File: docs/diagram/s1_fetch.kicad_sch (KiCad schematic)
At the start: 0 parts

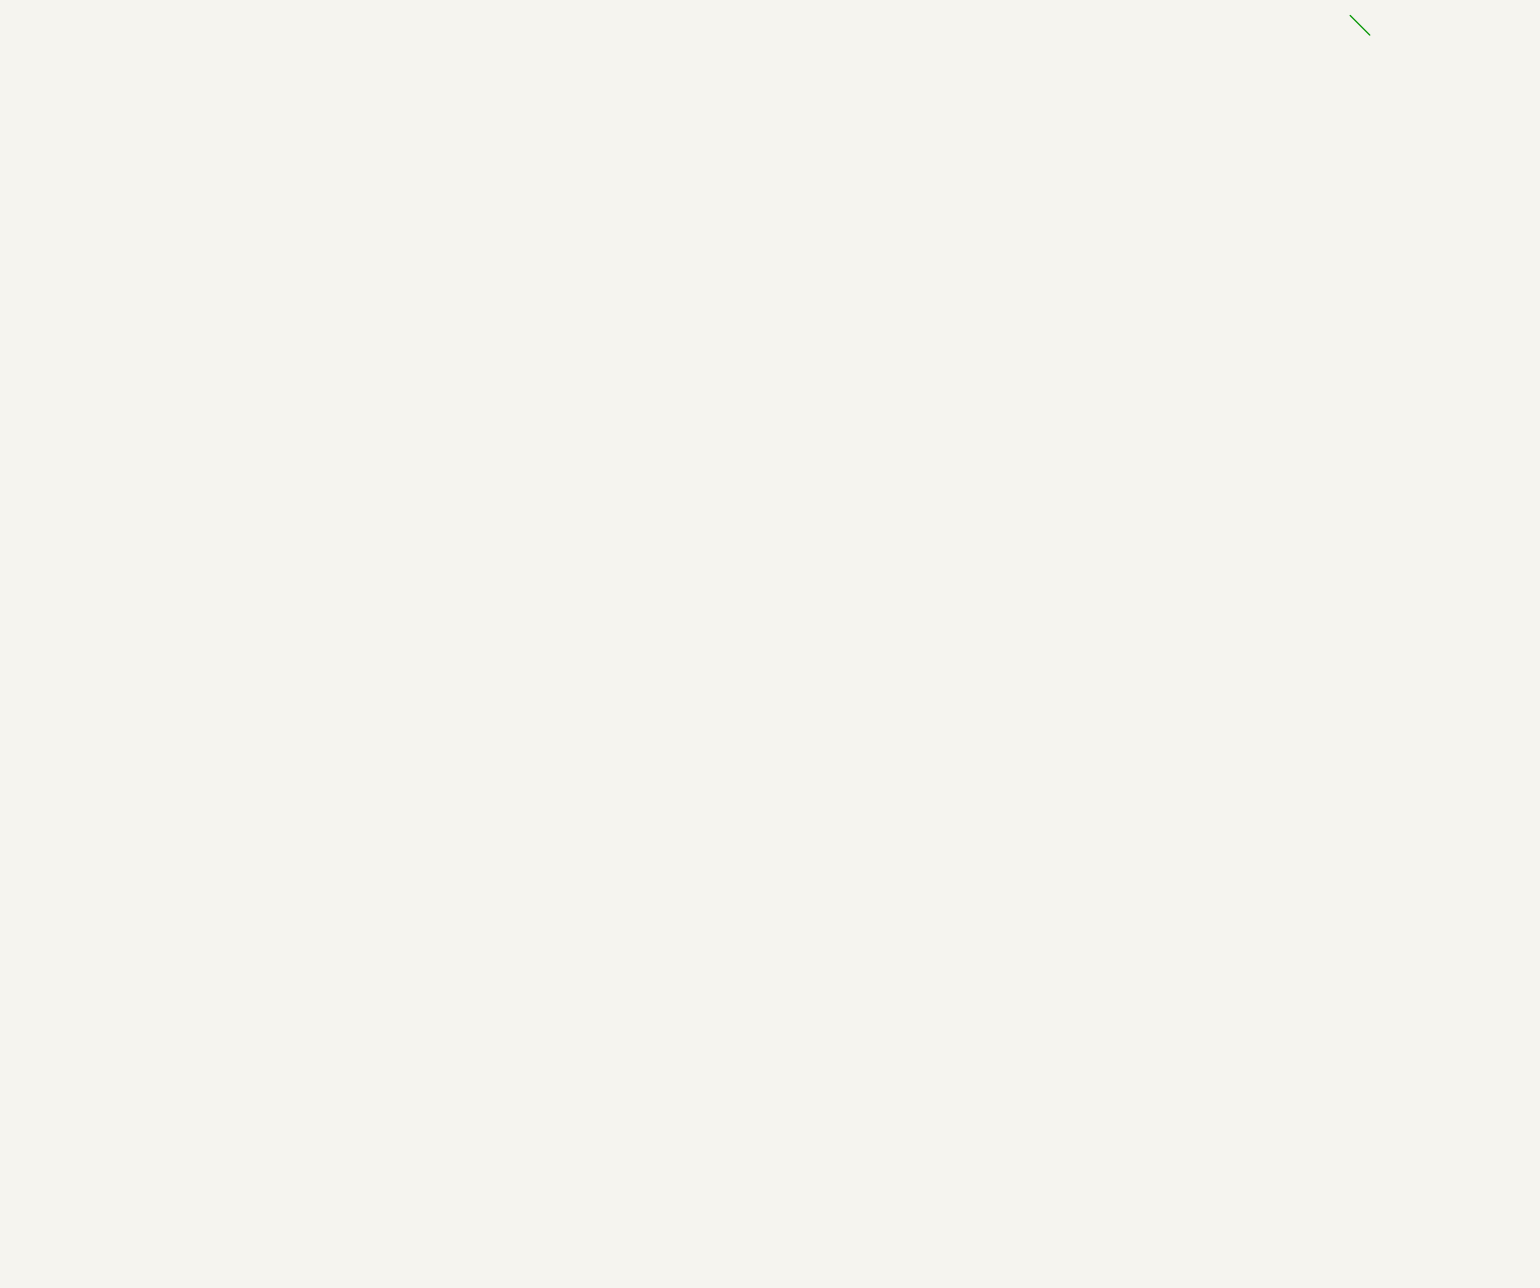
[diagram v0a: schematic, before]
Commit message: push
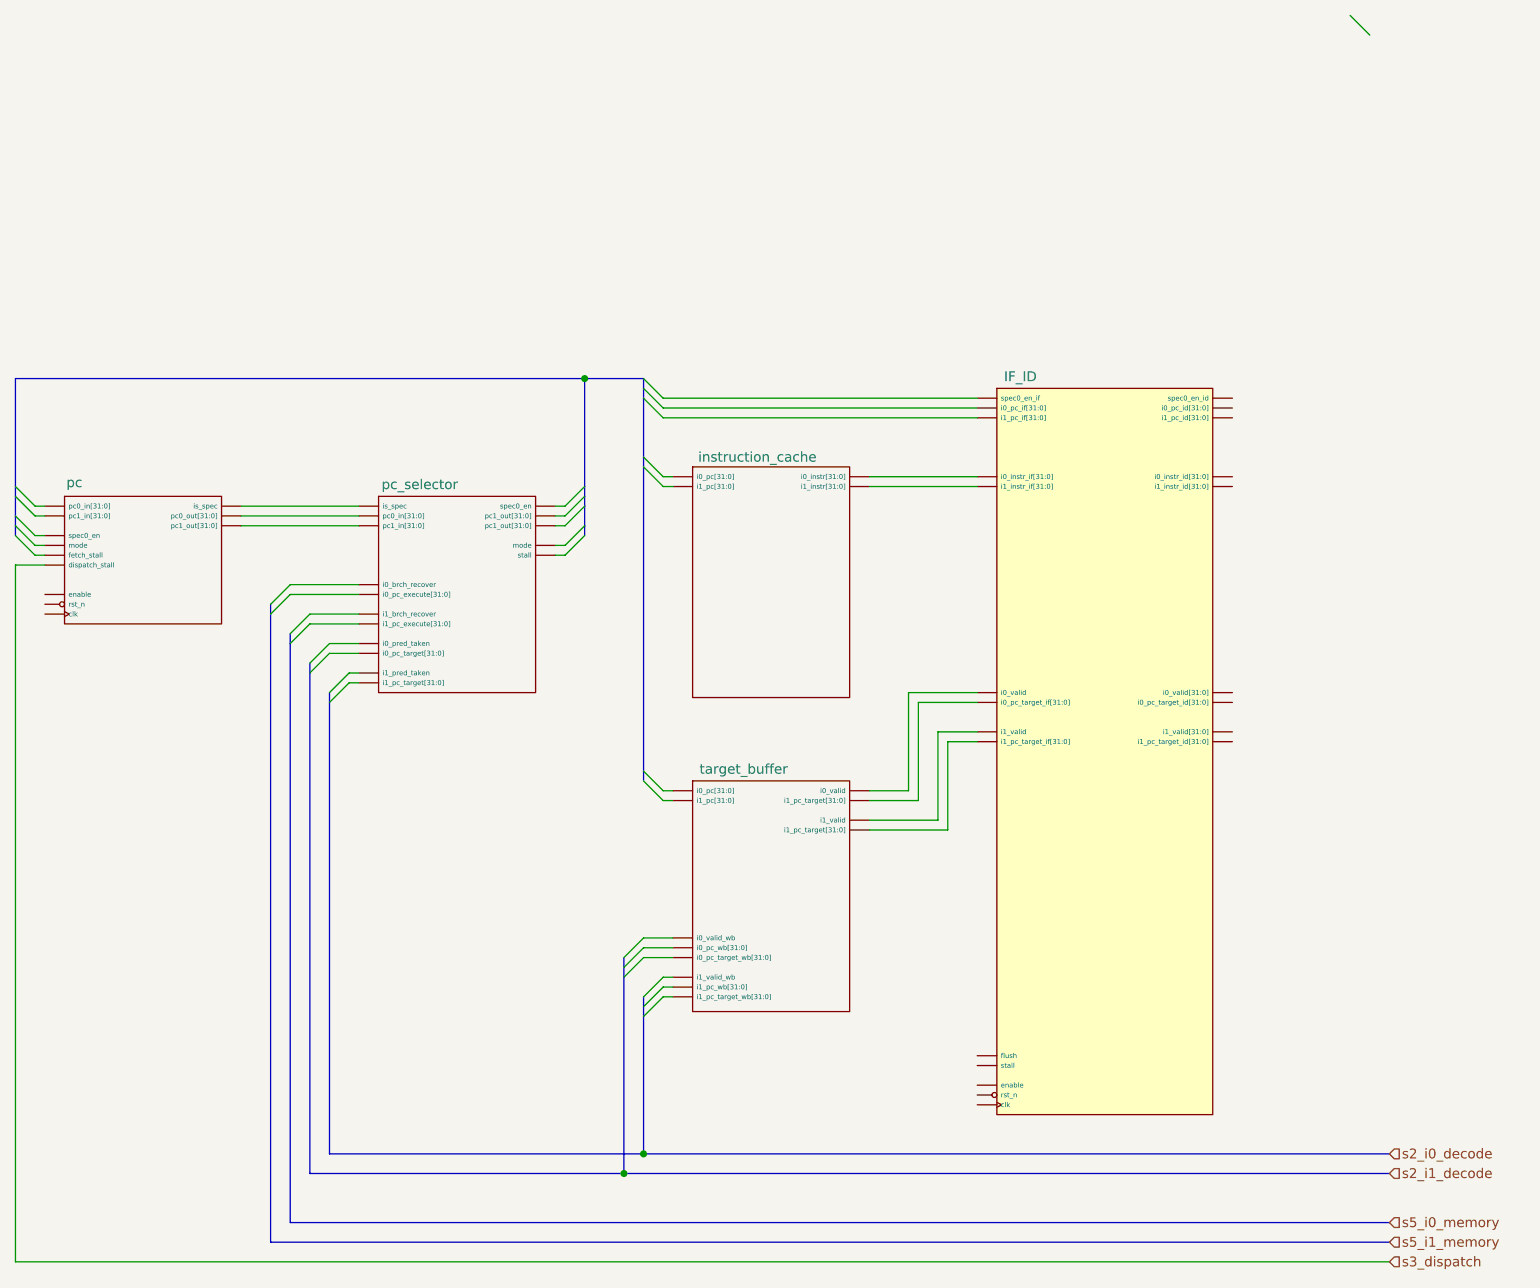
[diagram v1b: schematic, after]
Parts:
- added IF_ID: ~, symbol RV-DIS:IF_ID
- added instruction_cache: ~, symbol RV-DIS:instruction_cache
- added pc: ~, symbol RV-DIS:pc
- added pc_selector: ~, symbol RV-DIS:pc_selector
- added target_buffer: ~, symbol RV-DIS:target_buffer
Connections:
- new net: pc. (pc1_out[31:0]), pc_selector. (stall) (x3)
- new net: IF_ID. (i1_pc_target_id[31:0]), target_buffer. (i1_pc_target[31:0]) (x4)
- new net: IF_ID. (i1_pc_target_id[31:0]), instruction_cache. (i1_instr[31:0]) (x2)
- new net s3_dispatch: pc. (pc1_out[31:0])
